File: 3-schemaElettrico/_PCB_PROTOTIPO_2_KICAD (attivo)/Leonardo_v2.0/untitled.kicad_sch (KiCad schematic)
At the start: 1 part, among them U3 ESP32_NODEMCU

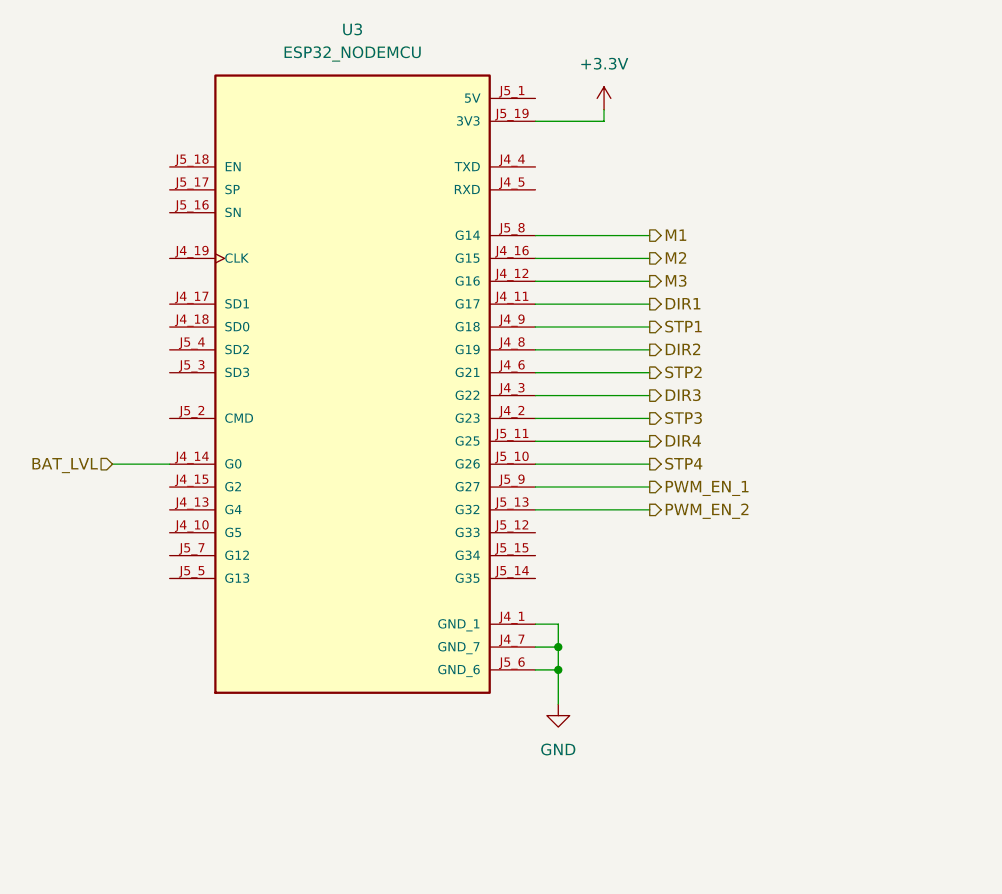
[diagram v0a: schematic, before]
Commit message: ok
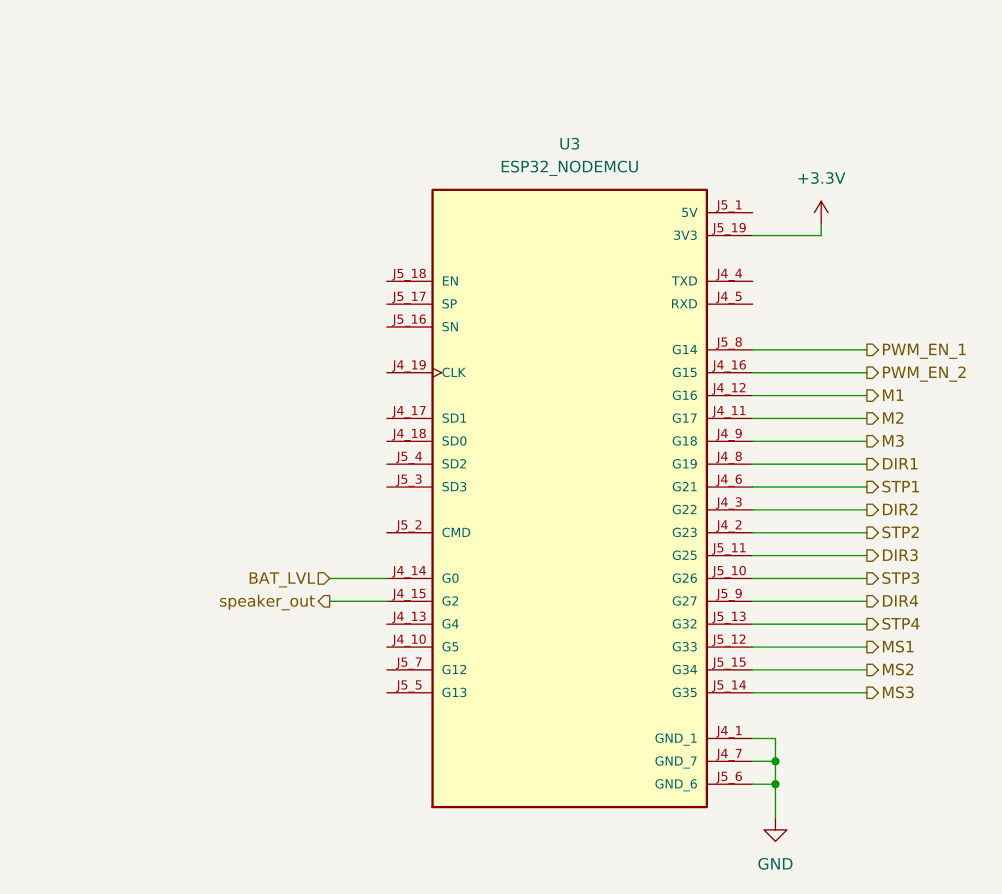
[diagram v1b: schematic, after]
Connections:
- net DIR1: now also U3.J4_8 (G19); no longer U3.J4_11 (G17)
- net DIR2: now also U3.J4_3 (G22); no longer U3.J4_8 (G19)
- net DIR3: now also U3.J5_11 (G25); no longer U3.J4_3 (G22)
- net DIR4: now also U3.J5_9 (G27); no longer U3.J5_11 (G25)
- net M1: now also U3.J4_12 (G16); no longer U3.J5_8 (G14)
- net M2: now also U3.J4_11 (G17); no longer U3.J4_16 (G15)
- net M3: now also U3.J4_9 (G18); no longer U3.J4_12 (G16)
- net PWM_EN_1: now also U3.J5_8 (G14); no longer U3.J5_9 (G27)
- net PWM_EN_2: now also U3.J4_16 (G15); no longer U3.J5_13 (G32)
- net STP1: now also U3.J4_6 (G21); no longer U3.J4_9 (G18)
- net STP2: now also U3.J4_2 (G23); no longer U3.J4_6 (G21)
- net STP3: now also U3.J5_10 (G26); no longer U3.J4_2 (G23)
- net STP4: now also U3.J5_13 (G32); no longer U3.J5_10 (G26)
- net speaker_out: now reaches U3.J4_15 (G2)
- net MS1: now reaches U3.J5_12 (G33)
- net MS3: now reaches U3.J5_14 (G35)
- net MS2: now reaches U3.J5_15 (G34)
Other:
- moved on the sheet: U3
